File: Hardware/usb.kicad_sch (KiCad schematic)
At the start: 24 parts, among them J14 USB_C_Receptacle_USB2.0, U12 SC2416H, U19 LTC4411, U8 INTERFACE-CP2102-GMR(QFN28)

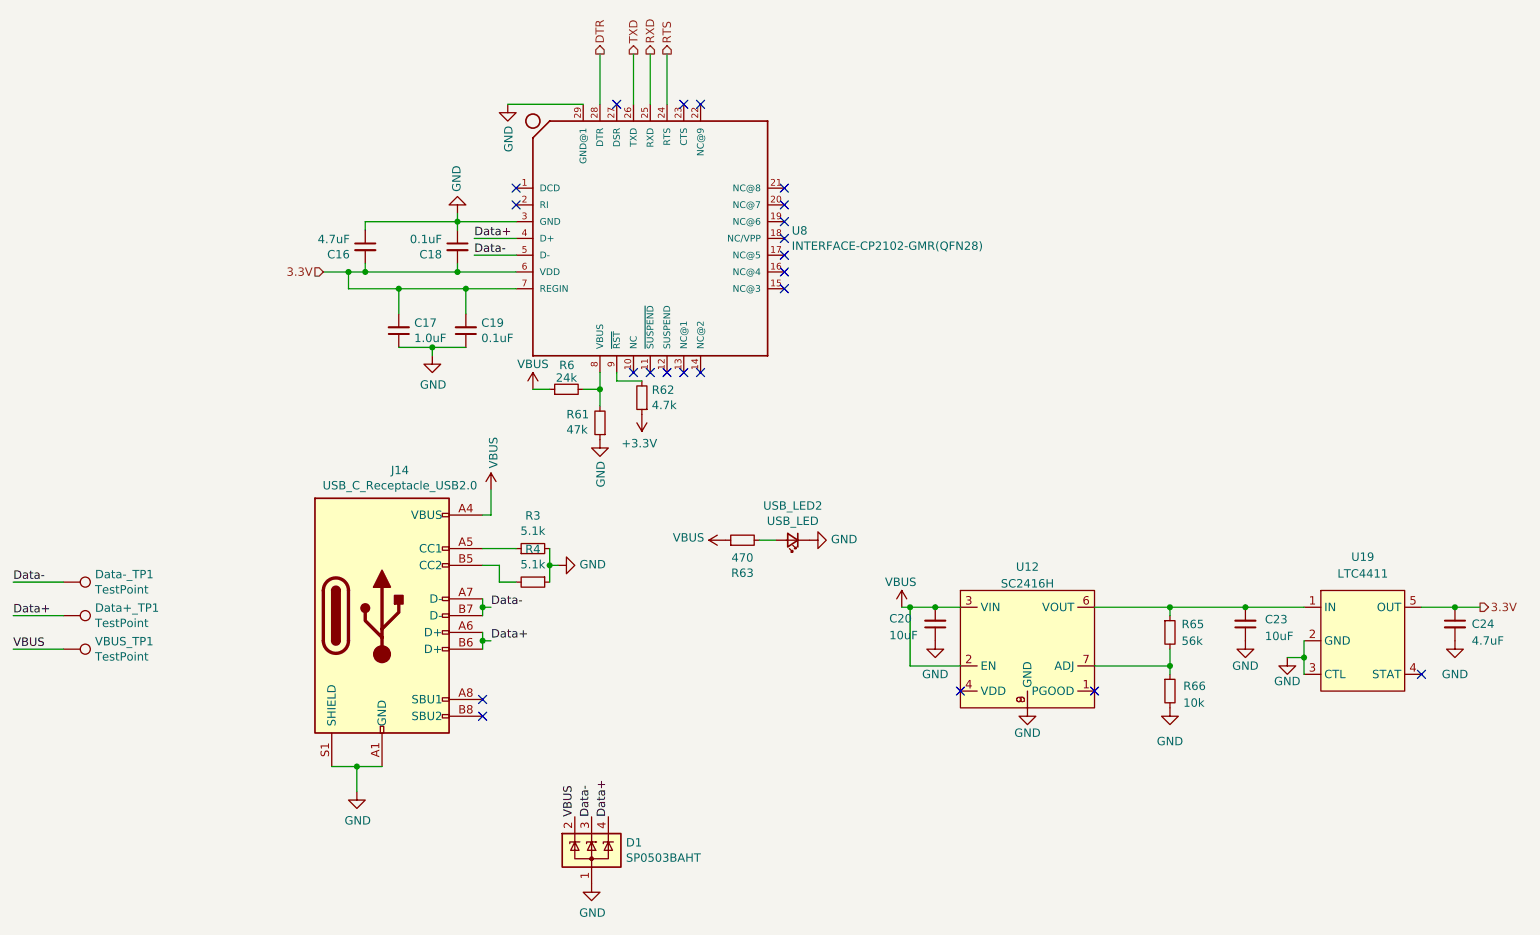
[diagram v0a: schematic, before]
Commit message: Start of Kermit Mini
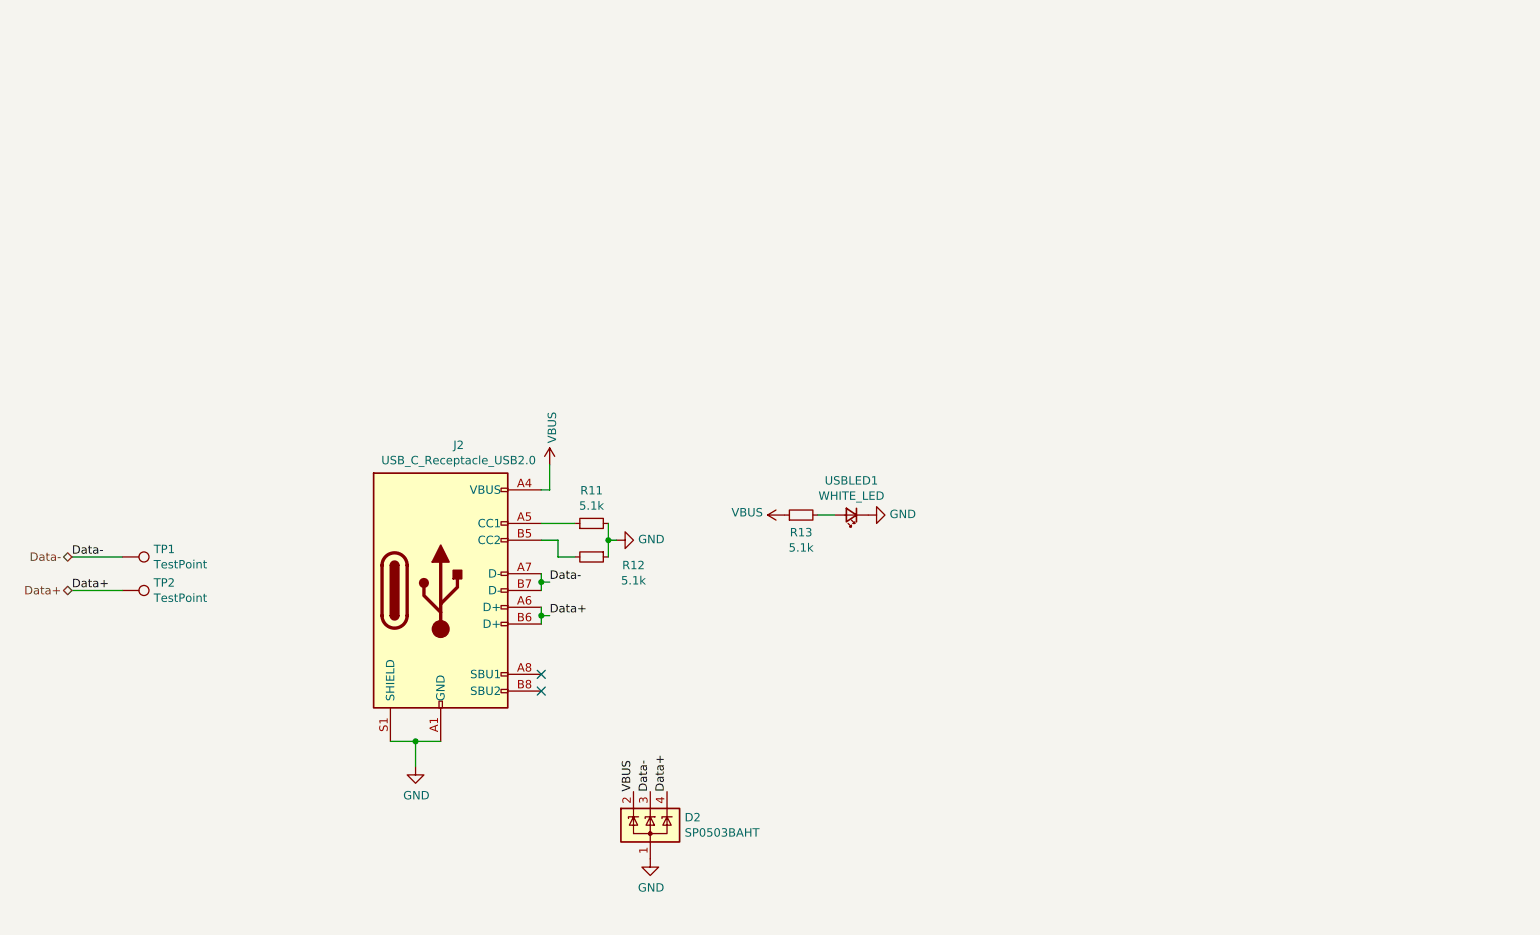
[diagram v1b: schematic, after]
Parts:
- removed C16, C24: 4.7uF, Capacitor_SMD:C_0603_1608Metric, symbol Device:C_Small
- removed C17: 1.0uF, Capacitor_SMD:C_0603_1608Metric, symbol Device:C_Small
- removed C18, C19: 0.1uF, Capacitor_SMD:C_0603_1608Metric, symbol Device:C_Small
- removed C20, C23: 10uF, Capacitor_SMD:C_0603_1608Metric, symbol Device:C_Small
- removed D1: SP0503BAHT, Package_TO_SOT_SMD:SOT-143, symbol Power_Protection:SP0503BAHT
- removed Data+_TP1, Data-_TP1, VBUS_TP1: TestPoint, TestPoint:TestPoint_Pad_D1.0mm, symbol Connector:TestPoint
- removed J14: USB_C_Receptacle_USB2.0, Connector_USB:USB_C_Receptacle_GCT_USB4085, symbol Connector:USB_C_Receptacle_USB2.0
- removed R3, R4: 5.1k, Resistor_SMD:R_0603_1608Metric, symbol Device:R_Small
- removed R6: 24k, Resistor_SMD:R_0603_1608Metric, symbol Device:R_Small
- removed R61: 47k, Resistor_SMD:R_0603_1608Metric, symbol Device:R_Small
- removed R62: 4.7k, Resistor_SMD:R_0603_1608Metric, symbol Device:R_Small
- removed R63: 470, Resistor_SMD:R_0603_1608Metric, symbol Device:R_Small
- removed R65: 56k, Resistor_SMD:R_0603_1608Metric, symbol Device:R_Small
- removed R66: 10k, Resistor_SMD:R_0603_1608Metric, symbol Device:R_Small
- removed U12: SC2416H, iclr:SOIC127P599X175-9N, symbol iclr:RT9025-25GSP
- removed U19: LTC4411, Package_TO_SOT_SMD:SOT-23-5, symbol iclr:LTC4411
- removed U8: INTERFACE-CP2102-GMR(QFN28), iclr:QFN28G_0.5-5X5MM, symbol iclr:INTERFACE-CP2102-GMR(QFN28)
- removed USB_LED2: USB_LED, LED_SMD:LED_0603_1608Metric, symbol Device:LED_Small
- added D2: SP0503BAHT, Package_TO_SOT_SMD:SOT-143, symbol Power_Protection:SP0503BAHT
- added J2: USB_C_Receptacle_USB2.0, Connector_USB:USB_C_Receptacle_Palconn_UTC16-G, symbol Connector:USB_C_Receptacle_USB2.0
- added R11, R12, R13: 5.1k, Resistor_SMD:R_0402_1005Metric, symbol Device:R_Small
- added TP1, TP2: TestPoint, TestPoint:TestPoint_Pad_D1.0mm, symbol Connector:TestPoint
- added USBLED1: WHITE_LED, Resistor_SMD:R_0402_1005Metric, symbol Device:LED_Small
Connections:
- net Data+: now also D2.4 (K), J2.A6 (D+), J2.B6 (D+), TP2.1
- net Data-: now also D2.3 (K), J2.A7 (D-), J2.B7 (D-), TP1.1
- net GND: now also D2.1 (A), J2.A1 (GND), J2.A12 (GND), J2.B1 (GND), J2.B12 (GND), J2.S1 (SHIELD), R11.2, R12.1, USBLED1.1 (K)
- net VBUS: now also D2.2 (K), J2.A4 (VBUS), J2.A9 (VBUS), J2.B4 (VBUS), J2.B9 (VBUS), R13.1
- new net: J2.B5 (CC2), R12.2
- new net: J2.A5 (CC1), R11.1
- new net: R13.2, USBLED1.2 (A)
- no-connect marks 22 -> 2
